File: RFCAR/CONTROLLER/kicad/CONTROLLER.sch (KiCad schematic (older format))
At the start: 17 parts, among them J1 Conn_01x08_Male, J2 Conn_01x07_Male, J3 Conn_01x06_Male, J4 Conn_01x01_Male, U1 LM1117-3.3, U2 L7805, U3 ATmega328P-PU, U4 ADG417BN, Y1 Crystal

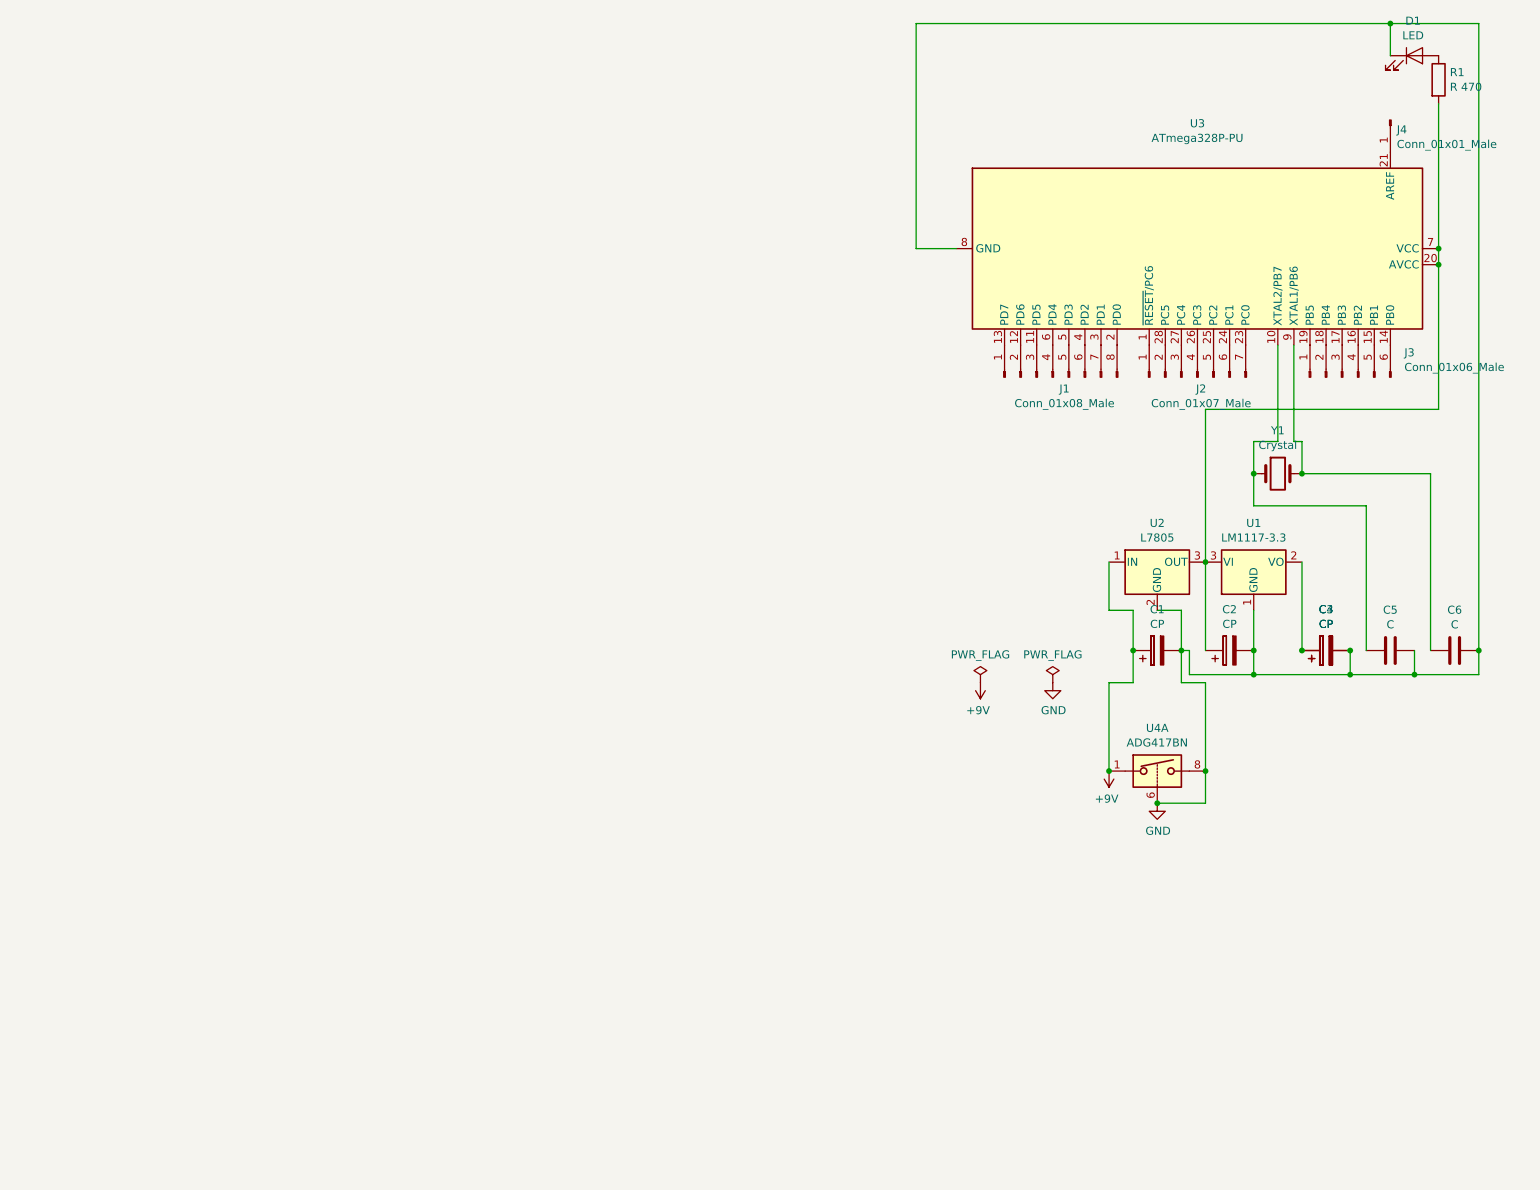
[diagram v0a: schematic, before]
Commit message: kicad
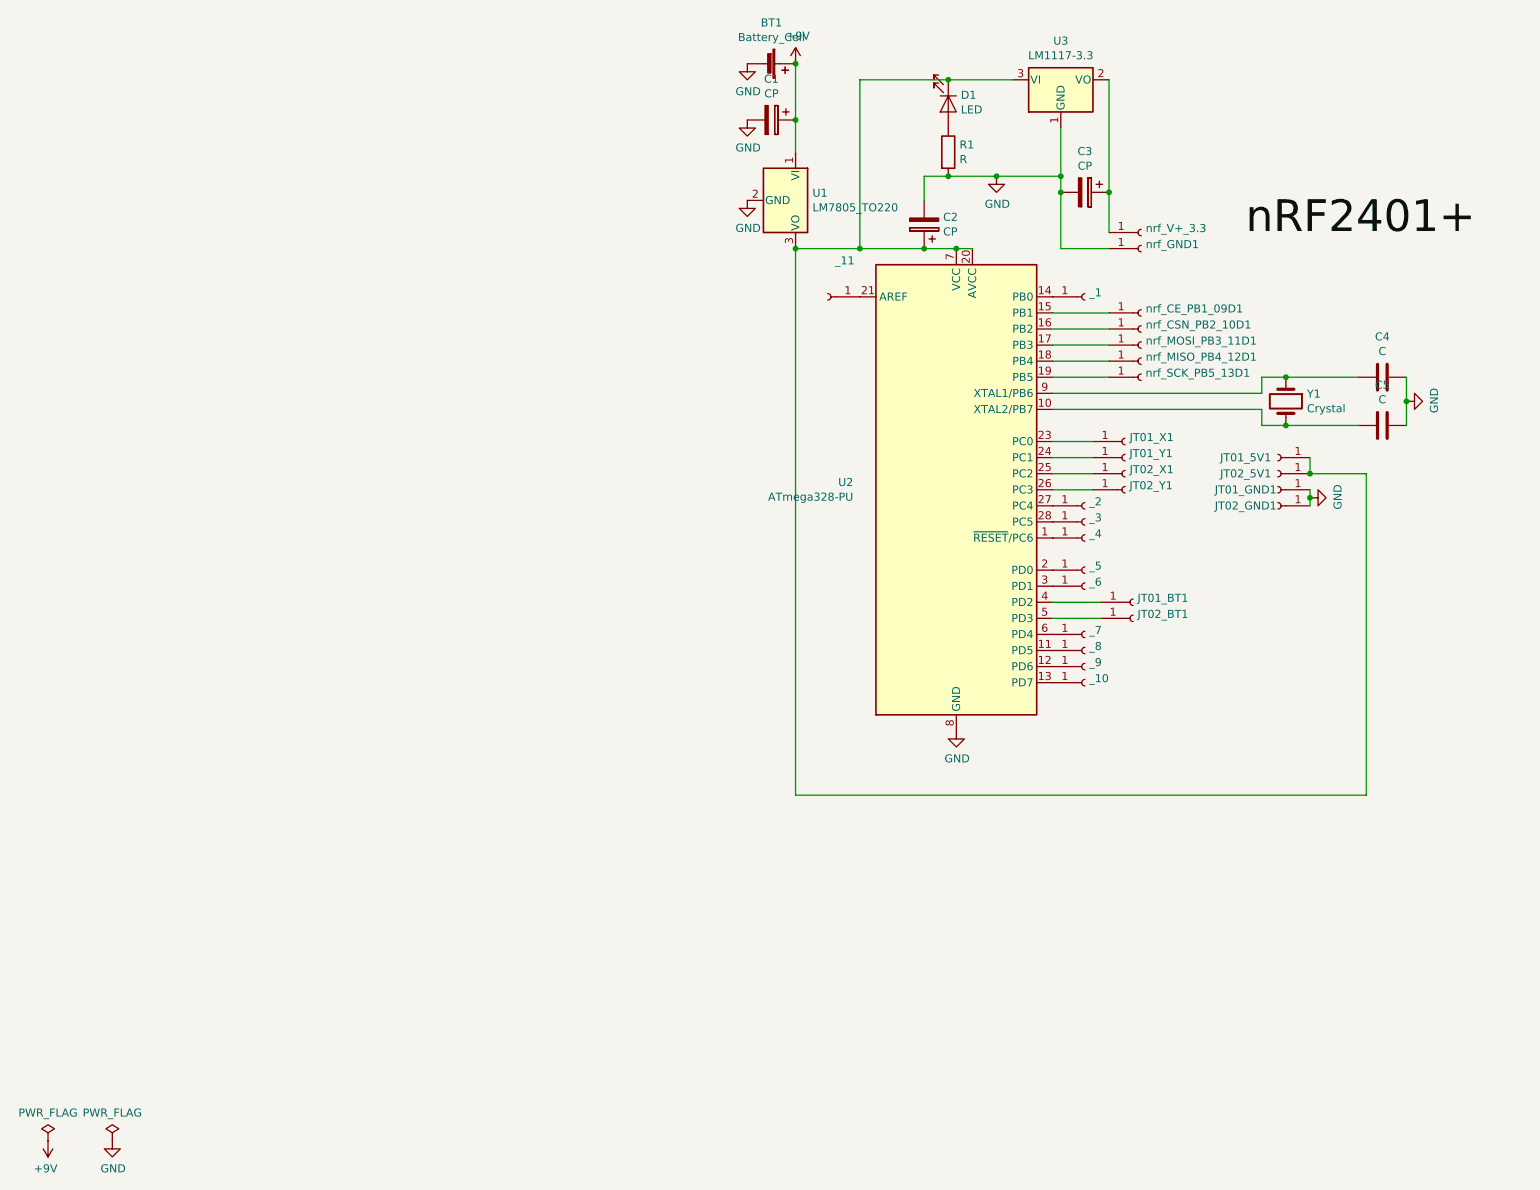
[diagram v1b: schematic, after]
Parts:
- removed C4: CP, symbol Device:CP
- removed C6: C, symbol Device:C
- removed J1: Conn_01x08_Male, symbol Connector:Conn_01x08_Male
- removed J2: Conn_01x07_Male, symbol Connector:Conn_01x07_Male
- removed J3: Conn_01x06_Male, symbol Connector:Conn_01x06_Male
- removed J4: Conn_01x01_Male, symbol Connector:Conn_01x01_Male
- removed U1: LM1117-3.3, symbol Regulator_Linear:LM1117-3.3
- removed U2: L7805, symbol Regulator_Linear:L7805
- removed U3: ATmega328P-PU, Package_DIP:DIP-28_W7.62mm, symbol MCU_Microchip_ATmega:ATmega328P-PU
- removed U4: ADG417BN, Package_DIP:DIP-8_W7.62mm, symbol Analog_Switch:ADG417BN
- added BT1: Battery_Cell, symbol Device:Battery_Cell
- added C4: C, Capacitor_THT:C_Axial_L3.8mm_D2.6mm_P7.50mm_Horizontal, symbol Device:C
- added JT01_5V1, JT01_BT1, JT01_GND1, JT01_X1, JT01_Y1, JT02_5V1, JT02_BT1, JT02_GND1, JT02_X1, JT02_Y1, _1, _10, _11, _2, _3, _4, _5, _6, _7, _8, _9, nrf_CE_PB1_09D1, nrf_CSN_PB2_10D1, nrf_GND1, nrf_MISO_PB4_12D1, nrf_MOSI_PB3_11D1, nrf_SCK_PB5_13D1, nrf_V+_3.3: (no value), Connector_PinHeader_2.00mm:PinHeader_1x01_P2.00mm_Vertical, symbol Connector:Conn_01x01_Female
- added U1: LM7805_TO220, Converter_DCDC:Converter_DCDC_TRACO_TSR-1_THT, symbol Regulator_Linear:LM7805_TO220
- added U2: ATmega328-PU, Package_DIP:DIP-28_W7.62mm, symbol MCU_Microchip_ATmega:ATmega328-PU
- added U3: LM1117-3.3, Converter_DCDC:Converter_DCDC_TRACO_TSR-1_THT, symbol Regulator_Linear:LM1117-3.3
- C1, C2, C3, C5: footprint (none) -> Capacitor_THT:C_Axial_L3.8mm_D2.6mm_P7.50mm_Horizontal
- R1: value R 470 -> R
- Y1: footprint (none) -> Crystal:Crystal_HC49-U_Vertical
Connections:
- net +9V: now also BT1.1 (+), U1.1 (VI)
- net GND: now also R1.2, BT1.2 (-), C4.1, JT01_GND1.1 (Pin_1), JT02_GND1.1 (Pin_1), U1.2 (GND), U2.22 (GND), U2.8 (GND), U3.1 (GND), nrf_GND1.1 (Pin_1); no longer D1.1 (K)
- net at C2.1: now also D1.1 (K), JT01_5V1.1 (Pin_1), JT02_5V1.1 (Pin_1), U1.3 (VO), U2.20 (AVCC), U2.7 (VCC), U3.3 (VI); no longer R1.2
- net at C3.1: now also U3.2 (VO), nrf_V+_3.3.1 (Pin_1)
- net at C5.2: now also Y1.2, U2.10 (XTAL2/PB7); no longer Y1.1
- new net: U2.1 (~RESET~/PC6), _4.1 (Pin_1)
- new net: U2.11 (PD5), _8.1 (Pin_1)
- new net: U2.12 (PD6), _9.1 (Pin_1)
- new net: U2.13 (PD7), _10.1 (Pin_1)
- new net: U2.14 (PB0), _1.1 (Pin_1)
- new net: U2.15 (PB1), nrf_CE_PB1_09D1.1 (Pin_1)
- new net: U2.16 (PB2), nrf_CSN_PB2_10D1.1 (Pin_1)
- new net: U2.17 (PB3), nrf_MOSI_PB3_11D1.1 (Pin_1)
- new net: U2.18 (PB4), nrf_MISO_PB4_12D1.1 (Pin_1)
- new net: U2.19 (PB5), nrf_SCK_PB5_13D1.1 (Pin_1)
- new net: U2.2 (PD0), _5.1 (Pin_1)
- new net: U2.21 (AREF), _11.1 (Pin_1)
- new net: JT01_X1.1 (Pin_1), U2.23 (PC0)
- new net: JT01_Y1.1 (Pin_1), U2.24 (PC1)
- new net: JT02_X1.1 (Pin_1), U2.25 (PC2)
- new net: JT02_Y1.1 (Pin_1), U2.26 (PC3)
- new net: U2.27 (PC4), _2.1 (Pin_1)
- new net: U2.28 (PC5), _3.1 (Pin_1)
- new net: U2.3 (PD1), _6.1 (Pin_1)
- new net: JT01_BT1.1 (Pin_1), U2.4 (PD2)
- new net: JT02_BT1.1 (Pin_1), U2.5 (PD3)
- new net: U2.6 (PD4), _7.1 (Pin_1)
- new net: C4.2, U2.9 (XTAL1/PB6), Y1.1
